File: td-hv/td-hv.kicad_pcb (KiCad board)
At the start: 2 copper layers, 100 x 60 mm, 39 parts, among them J1 Conn_01x06_Male, Q1 IMBF170R450M1XTMA1, U1 UCC2801, U2 TL081, U3 LM2903

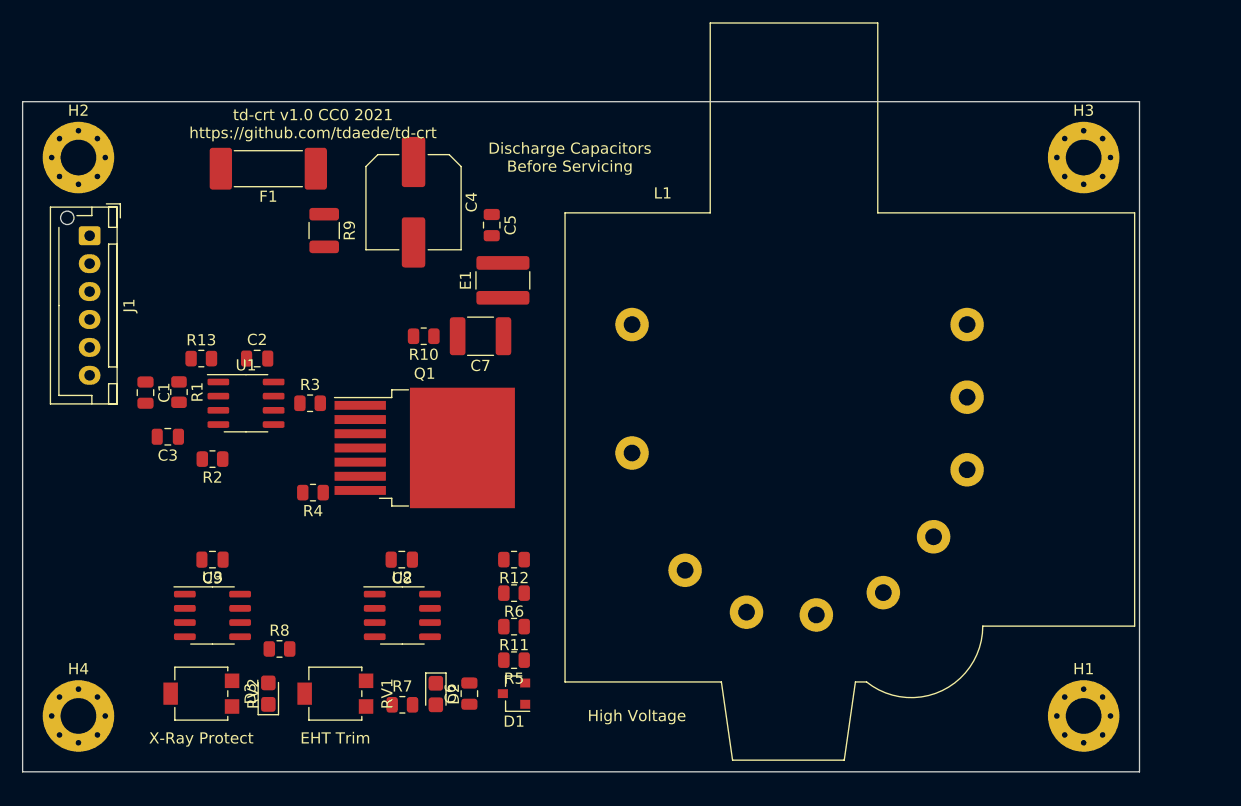
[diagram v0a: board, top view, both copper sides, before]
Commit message: some td-hv layout
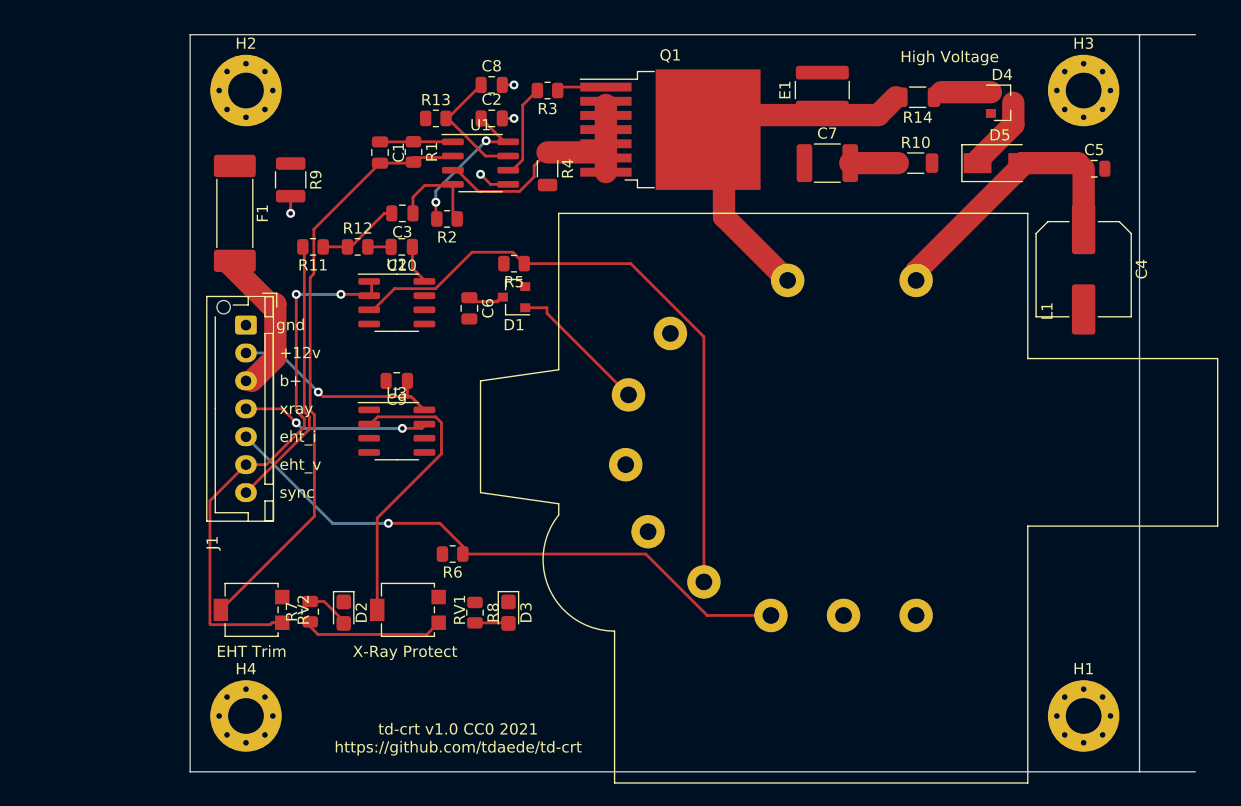
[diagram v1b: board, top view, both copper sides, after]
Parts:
- added C10: 0.1uF, Capacitor_SMD:C_0805_2012Metric, F.Cu at (-69.0, -17.0)
- added D4: BAS21, Package_TO_SOT_SMD:SOT-23, F.Cu at (-15.3, -29.9)
- added D5: SMAJ400ALFCT-ND, Diode_SMD:D_SMA, F.Cu at (-15.5, -24.5)
- added R14: 50, Resistor_SMD:R_1206_3216Metric, F.Cu at (-22.9, -30.4)
- J1: value Conn_01x06_Male -> Conn_01x07_Male; footprint Connector_JST:JST_XH_B6B-XH-AM_1x06_P2.50mm_Vertical -> Connector_JST:JST_XH_B7B-XH-AM_1x07_P2.50mm_Vertical
- R10, R4: footprint Resistor_SMD:R_0805_2012Metric -> Resistor_SMD:R_1206_3216Metric
- R11: value 100k -> 120
- R12: value 100 -> 50
- U2: value TL081 -> TLC272
- moved C4 60.3 mm to (-8.00, -15.0)
- moved C5 54.2 mm to (-7.05, -24.0), turned to 0 degrees
- moved R10 46.7 mm to (-23.0, -24.5), turned to 0 degrees
- moved C8 43.3 mm to (-61.0, -31.5), turned to 0 degrees
- moved R11 38.5 mm to (-77.0, -17.0)
- moved Q1 36.0 mm to (-45.0, -27.5)
- moved R4 35.8 mm to (-56.0, -24.0), turned to 270 degrees
- moved D1 35.5 mm to (-59.0, -12.5)
- moved R5 35.5 mm to (-59.0, -15.5)
- moved R3 35.2 mm to (-56.0, -31.0), turned to 180 degrees
- moved C7 34.7 mm to (-30.9, -24.5), turned to 0 degrees
- moved C6 34.5 mm to (-63.0, -11.5), turned to 270 degrees
- moved E1 33.3 mm to (-31.4, -31.0)
- moved R12 31.3 mm to (-73.0, -17.0), turned to 0 degrees
- moved C1 30.1 mm to (-71.0, -25.4)
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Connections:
- net Net-(C7-Pad2) renamed /snubber_node
- net Net-(F1-Pad2) renamed /vbus_in
- C3 pad 2: GND -> Net-(C3-Pad2)
- C8 pad 1: +12V -> Net-(C8-Pad1)
- R11 pad 1: Net-(L1-Pad7) -> Net-(C3-Pad2)
- R11 pad 2: GND -> /sync_in
- R12 pad 1: /eht_current -> Net-(C3-Pad2)
- R13 pad 2: Net-(R13-Pad2) -> Net-(C8-Pad1)
- R2 pad 2: GND -> /ucc3801_ref
- U1 pad 7: Net-(R13-Pad2) -> Net-(C8-Pad1)
- U2 pad 1: Net-(U2-Pad1) -> /eht_voltage
- U2 pad 5: Net-(U2-Pad5) -> (no net)
- U2 pad 6: /eht_voltage -> (no net)
- U2 pad 7: +12V -> (no net)
- U2 pad 8: Net-(U2-Pad8) -> +12V
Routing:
- net Net-(L1-Pad7): track 0.00 -> 57.2 mm
- net /eht_current: track 0.00 -> 54.5 mm, vias 0 -> 1
- net /fb: track 0.00 -> 53.4 mm
- net /eht_voltage: track 0.00 -> 49.0 mm, vias 0 -> 2
- net /sw: track 0.00 -> 33.2 mm
- net Net-(RV1-Pad2): track 0.00 -> 26.2 mm
- net VBUS: track 0.00 -> 24.8 mm
- net /sync_in: track 0.00 -> 24.6 mm
- net +12V: track 0.00 -> 24.2 mm, vias 0 -> 1
- net /cs: track 0.00 -> 22.5 mm
- net /~xray_protect: track 0.00 -> 16.8 mm, vias 0 -> 2
- net Net-(C6-Pad1): track 0.00 -> 16.3 mm
- net /ucc3801_ref: track 0.00 -> 13.6 mm, vias 0 -> 2
- net /vbus_in: track 0.00 -> 13.4 mm
- net Net-(D1-Pad1): track 0.00 -> 12.8 mm
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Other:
- board size 100 x 60 mm -> 90 x 66 mm
- net class hv added: clearance 1.5, trace_width 0.25, via_dia 0.8, via_drill 0.4
- board text added: "+12v"
- board text added: "b+"
- board text added: "eht_i"
- board text added: "eht_v"
- board text added: "gnd"
- board text added: "sync"
- board text added: "xray"
- board text removed: "Discharge Capacitors Before Servicing"
